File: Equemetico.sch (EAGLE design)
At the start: 21 parts, among them IC1 RASPBERRY_PI_ZERO_W_(V1.3), K1 SRD-05VDC-SL-C, K2 SRD-05VDC-SL-C, K3 SRD-05VDC-SL-C, K4 SRD-05VDC-SL-C, K5 SRD-05VDC-SL-C

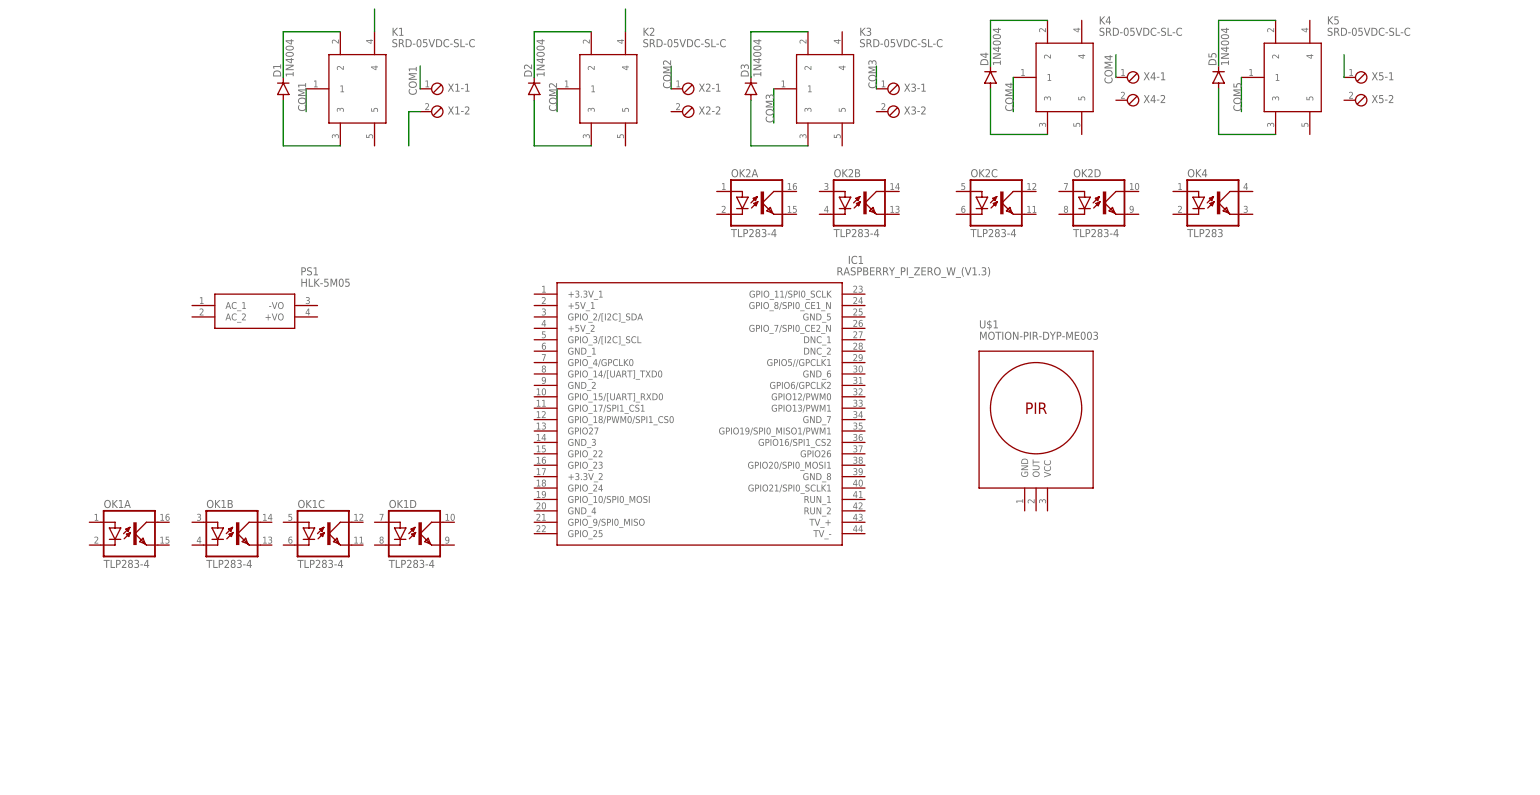
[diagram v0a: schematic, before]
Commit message: Coenexion de relevadores
Relevadores conectados
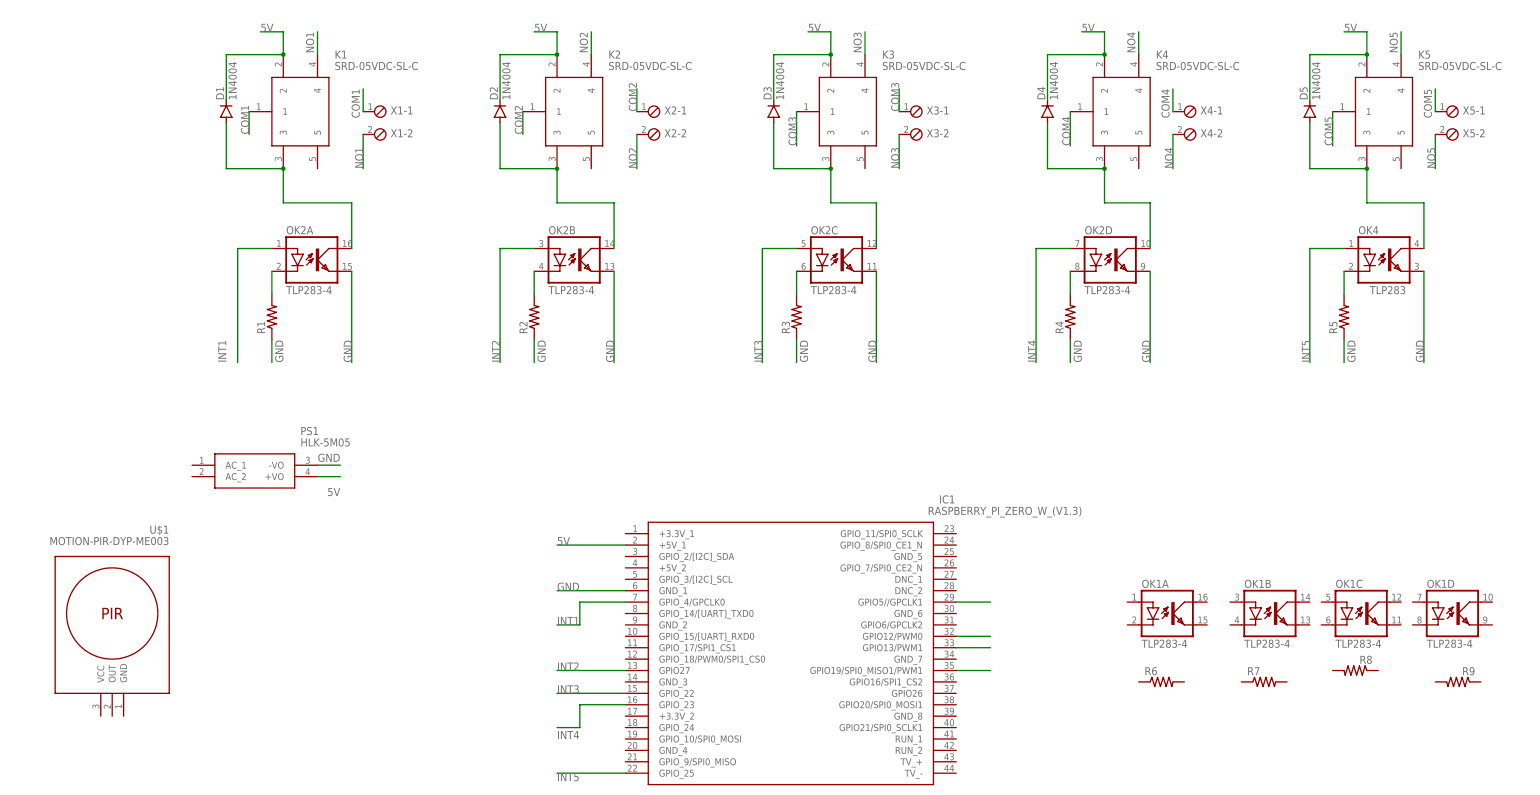
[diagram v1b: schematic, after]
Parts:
- added R1, R2, R3, R4, R5, R6, R7, R8, R9: (no value), rcl:R-US_R0402
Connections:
- removed net N$1: D1.C, K1.2
- removed net N$2: D1.A, K1.3
- removed net N$3: D2.C, K2.2
- removed net N$4: D2.A, K2.3
- removed net N$9: D5.C, K5.2
- new net 5V: D1.C, D2.C, D3.C, D4.C, D5.C, IC1.+5V_1, K1.2, K2.2, K3.2, K4.2, K5.2, PS1.+VO
- new net GND: IC1.GND_1, OK2A.EMIT, OK2B.EMIT, OK2C.EMIT, OK2D.EMIT, OK4.EMIT, PS1.-VO, R1.1, R2.1, R3.1, R4.1, R5.1
- new net INT1: IC1.GPIO_4/GPCLK0, OK2A.A
- new net INT2: IC1.GPIO27, OK2B.A
- new net INT3: IC1.GPIO_22, OK2C.A
- new net INT4: IC1.GPIO_23, OK2D.A
- new net INT5: IC1.GPIO_25, OK4.A
- new net N$14: OK4.C, R5.2
- new net N$30: D5.A, K5.3, OK4.COL
- new net N$32: D4.A, K4.3, OK2D.COL
- new net N$33: D3.A, K3.3, OK2C.COL
- new net N$34: D2.A, K2.3, OK2B.COL
- new net N$35: D1.A, K1.3, OK2A.COL
- new net NO1: K1.4, X1-2.1
- new net NO2: K2.4, X2-2.1
- new net NO3: K3.4, X3-2.1
- new net NO4: K4.4, X4-2.1
- new net NO5: K5.4, X5-2.1
- net N$10: now also OK2A.C, R1.2; no longer D5.A, K5.3
- net N$11: now also OK2B.C, R2.2; no longer K1.4
- net N$12: now also OK2C.C, R3.2; no longer X1-2.1
- net N$13: now also OK2D.C, R4.2; no longer K2.4
- net N$5: now also IC1.GPIO19/SPI0_MISO1/PWM1; no longer D3.C, K3.2
- net N$6: now also IC1.GPIO13/PWM1; no longer D3.A, K3.3
- net N$7: now also IC1.GPIO12/PWM0; no longer D4.C, K4.2
- net N$8: now also IC1.GPIO5//GPCLK1; no longer D4.A, K4.3
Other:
- moved on the sheet: D1, D2, D3, D4, D5, IC1, K1, K2, K3, K4, K5, OK1A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
